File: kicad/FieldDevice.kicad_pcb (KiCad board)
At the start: 2 copper layers, 47 x 41.9 mm, 34 parts, among them P201 Positive, P202 Negative, Q301 Q_PMOS_GSD, SW301 SW_PUSH, U101 Teensy-3.2, U501 DS7505

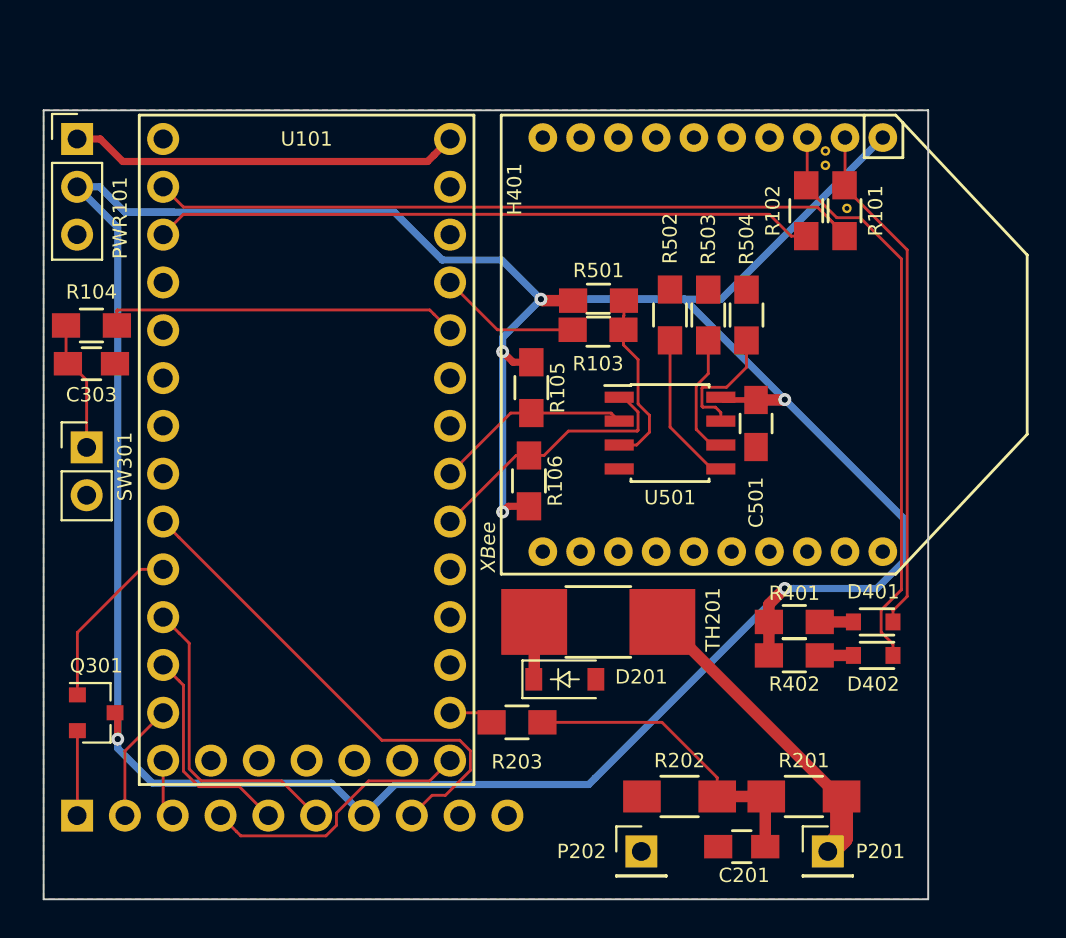
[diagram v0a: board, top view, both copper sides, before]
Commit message: More changes to the layout for the Power System integration
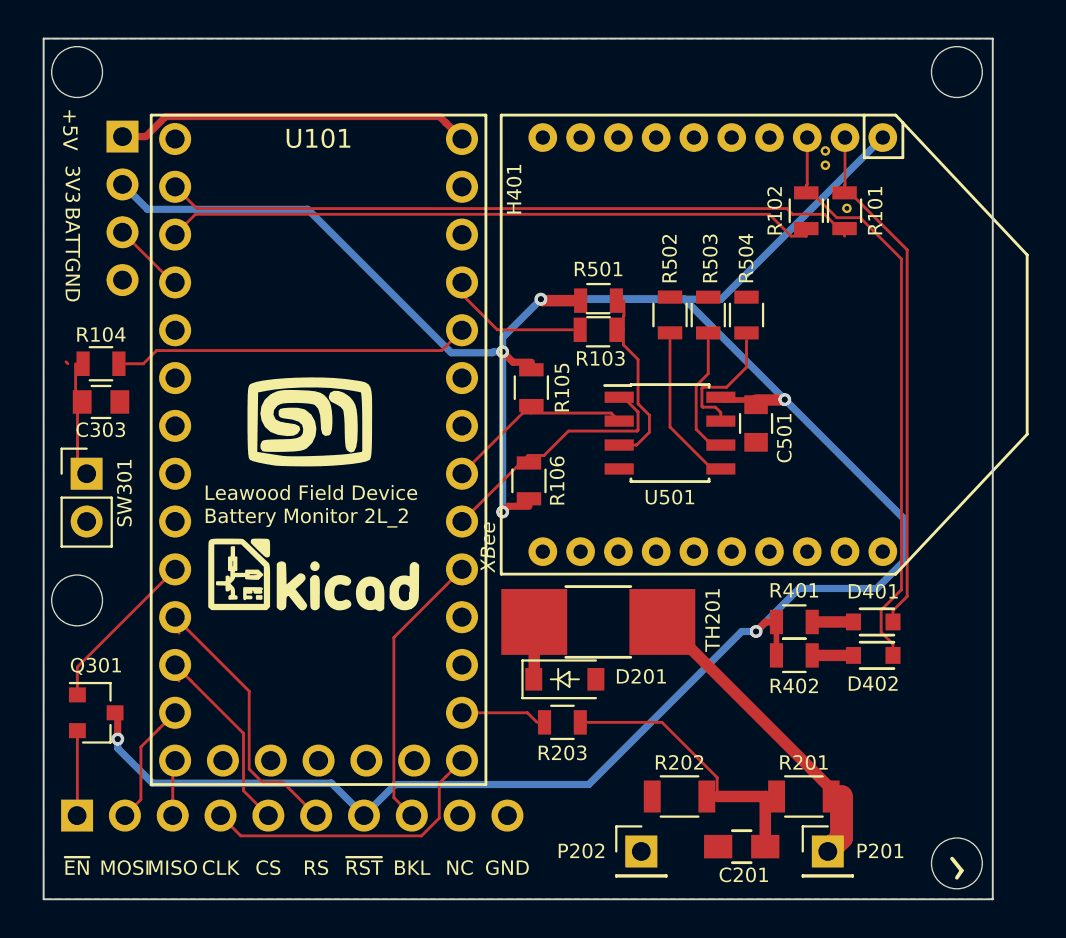
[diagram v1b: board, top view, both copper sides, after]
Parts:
- added G***: LOGO, FieldDevice_Footprints:KiCad-Logo, B.Cu at (43.6, 75.4)
- added G***: LOGO, FieldDevice_Footprints:MyBasic_rounded_50_1, B.Cu at (43.3, 67.3)
- added G***: LOGO, FieldDevice_Footprints:MyBasic_rounded_50_1, F.Cu at (43.3, 67.3)
- added G***: LOGO, FieldDevice_Footprints:KiCad-Logo, F.Cu at (43.6, 75.4)
- added REF**: MountingHole_2.7mm_M2.5, Mounting_Holes:MountingHole_2.7mm_M2.5, F.Cu at (31.1, 77.0)
- added REF**: MountingHole_2.7mm_M2.5, Mounting_Holes:MountingHole_2.7mm_M2.5, F.Cu at (77.9, 48.9)
- added REF**: MountingHole_2.7mm_M2.5, Mounting_Holes:MountingHole_2.7mm_M2.5, F.Cu at (77.7, 90.8)
- added REF**: MountingHole_2.7mm_M2.5, Mounting_Holes:MountingHole_2.7mm_M2.5, F.Cu at (31.0, 48.8)
- C303, C501: footprint Capacitors_SMD:C_0805_HandSoldering -> Capacitors_SMD:C_0805
- PWR101: footprint Pin_Headers:Pin_Header_Straight_1x03_Pitch2.54mm -> Pin_Headers:Pin_Header_Angled_1x04_Pitch2.54mm; moved to B.Cu
- R101, R102, R103, R104, R105, R106, R203, R401, R402, R501, R502, R503, R504: footprint Resistors_SMD:R_0805_HandSoldering -> Resistors_SMD:R_0805
- R201, R202: footprint Resistors_SMD:R_1206_HandSoldering -> Resistors_SMD:R_1206
- moved PWR101 2.42 mm to (33.4, 52.2), turned to 180 degrees
- moved R203 2.41 mm to (56.8, 83.3)
- moved R104 2.09 mm to (32.3, 64.3)
- moved C303 2.09 mm to (32.3, 66.3)
- moved SW301 1.40 mm to (31.5, 70.1)
- moved U101 0.63 mm to (43.8, 67.6)
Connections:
- PWR101 pad 3: GND -> /BATT
- U101 pad 17: (no net) -> /BACKLIGHT
- U101 pad 2: (no net) -> /BATT
- U101 pad 7: /BACKLIGHT -> (no net)
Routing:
- net /3V3: track 183.3 -> 146.5 mm
- net /BACKLIGHT: track 26.5 -> 15.0 mm
- net /BATT: track 0.00 -> 3.90 mm
- net Net-(C201-Pad1): track 16.8 -> 14.4 mm
- net Net-(R101-Pad2): track 38.6 -> 36.7 mm
- net /5V: track 20.8 -> 19.0 mm
- net /ANLG_1: track 2.42 -> 4.19 mm
- net /SPI_CLK: track 14.7 -> 16.0 mm
- net /REG_SEL: track 16.4 -> 15.5 mm
- net /Display: track 7.00 -> 6.09 mm
- net /SPI_CS: track 12.0 -> 11.3 mm
- net Net-(R102-Pad2): track 35.2 -> 34.6 mm
- net /I2C_SDA: track 14.3 -> 13.7 mm
- net /I2C_SCK: track 11.0 -> 10.3 mm
- net /MISO: track 3.13 -> 3.69 mm
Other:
- board size 47 x 41.9 mm -> 50.4 x 45.7 mm
- board text added: "+5V"
- board text added: "3V3"
- board text added: "BATT"
- board text added: "BKL"
- board text added: "CLK"
- board text added: "CS"
- board text added: "GND"
- board text added: "Leawood Field Device Battery Monitor 2L_2"
- board text added: "MISO"
- board text added: "MOSI"
- board text added: "NC"
- board text added: "RS"
- board text added: "~EN"
- board text added: "~RST"
